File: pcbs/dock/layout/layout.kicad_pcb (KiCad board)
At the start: 2 copper layers, 37 parts, among them J1 53047-0210, J2 ?, J3 53047-0610, U1 MCP73831T-2ACI/OT, U2 AP2112K-1.8TRG1, U3 AMS1117-3.3, U4 W25Q16JVSSIQ, U5 RP2040, U6 ?, Y1 12MHz 10pF

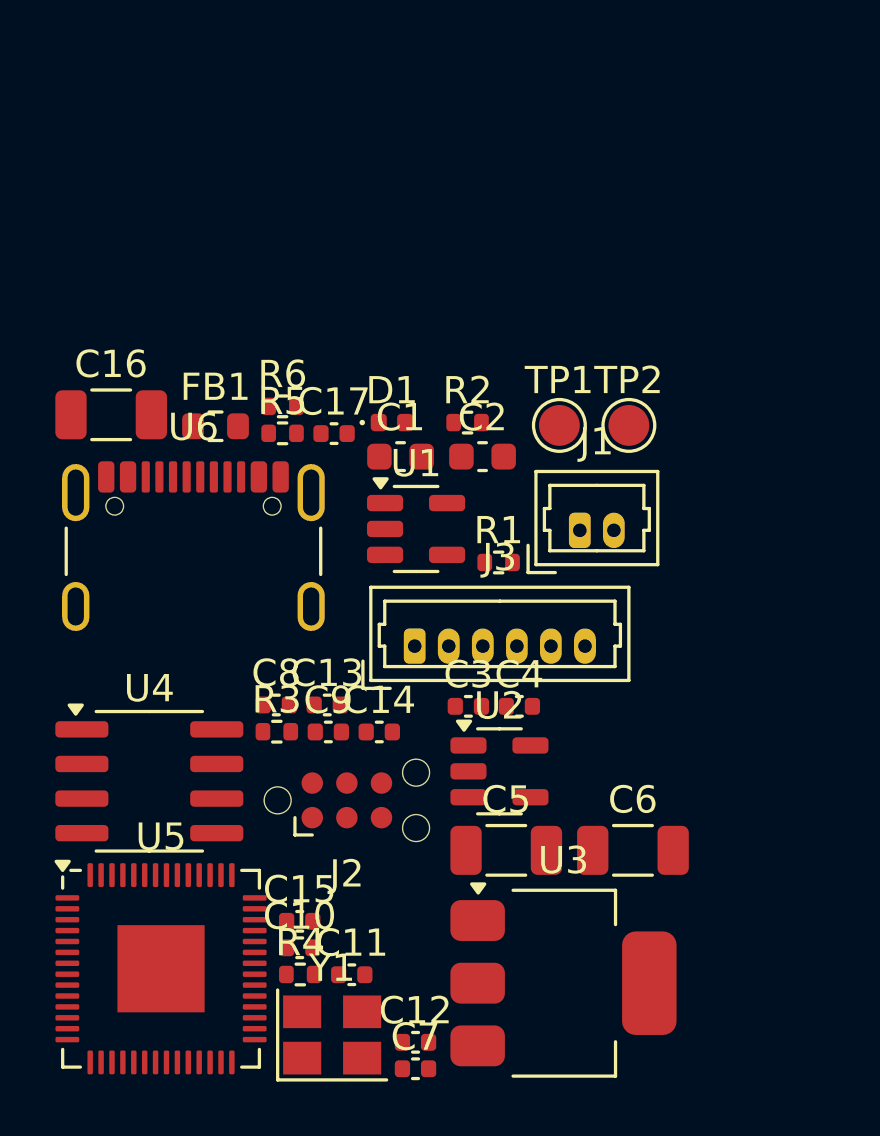
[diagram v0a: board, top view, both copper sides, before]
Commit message: cleanup
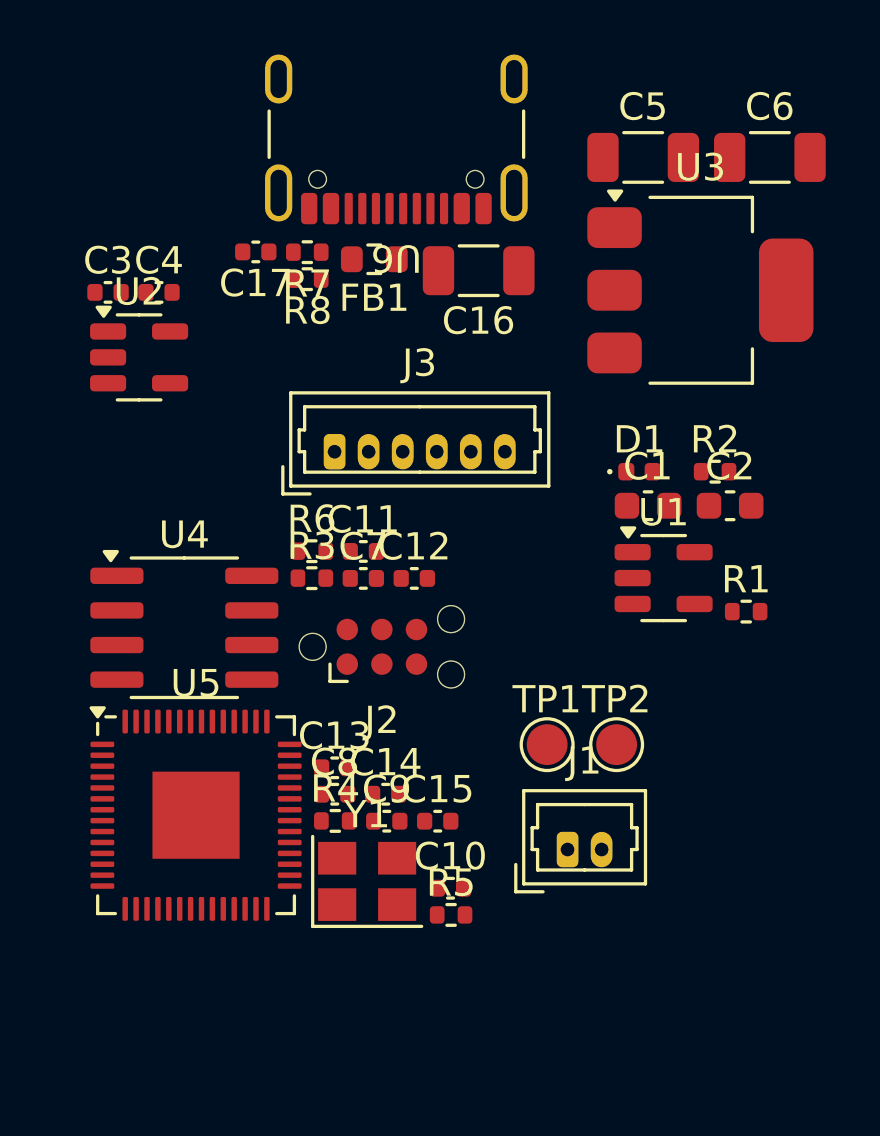
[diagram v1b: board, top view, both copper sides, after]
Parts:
- added R7: 5.1k 1%, R_0402_1005Metric:R_0402_1005Metric, F.Cu at (146.1, 87.4)
- added R8: 5.1k 1%, R_0402_1005Metric:R_0402_1005Metric, F.Cu at (146.1, 88.4)
- C9: value 100nF 10V -> 100nF 6.3V
- R4: value 10k -> 27
- R5: value 5.1k 1% -> 27
- R6: value 5.1k 1% -> 10k
- U4: value W25Q16JVSSIQ -> MX25R3235FM1IH0
- moved C6 25.9 mm to (163.1, 83.9)
- moved U3 25.9 mm to (160.6, 88.8)
- moved C5 25.9 mm to (158.4, 83.9)
- moved U2 20.1 mm to (139.9, 91.2)
- moved C3 20.1 mm to (138.8, 88.9)
- moved C4 20.1 mm to (140.7, 88.9)
- moved U6 18.8 mm to (149.4, 82.1), turned to 180 degrees
- moved R5 18.7 mm to (151.4, 111.7)
- moved C7 18.1 mm to (148.2, 99.3)
- moved C12 17.0 mm to (150.1, 99.3)
- moved C11 15.5 mm to (148.2, 98.4)
- moved C16 14.5 mm to (152.4, 88.1), turned to 180 degrees
- moved TP2 11.7 mm to (157.5, 105.5)
- moved J1 11.7 mm to (155.7, 109.3)
- moved TP1 11.7 mm to (154.9, 105.5)
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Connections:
- net ldo1.NC renamed ldo1v8.NC
- C9 pad 1: VDD_3V3 -> VDD_1V8
- R3 pad 2: VDD_3V3 -> VDD_1V8
- R4 pad 1: probe.QSPI_SD2_3 -> probe.usb_dm_mcu
- R4 pad 2: VDD_3V3 -> USB_DM
- R5 pad 1: usb.CC1 -> probe.usb_dp_mcu
- R5 pad 2: GND -> USB_DP
- R6 pad 1: usb.CC2 -> probe.QSPI_SD2_3
- R6 pad 2: GND -> VDD_1V8
- U4 pad 8: VDD_3V3 -> VDD_1V8
- U5 pad 46: USB_DN -> probe.usb_dm_mcu
- U5 pad 47: USB_DP -> probe.usb_dp_mcu
- U6 pad A7: USB_DN -> USB_DM
- U6 pad B7: USB_DN -> USB_DM
